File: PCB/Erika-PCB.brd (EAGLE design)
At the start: 100 x 80 mm, 11 parts

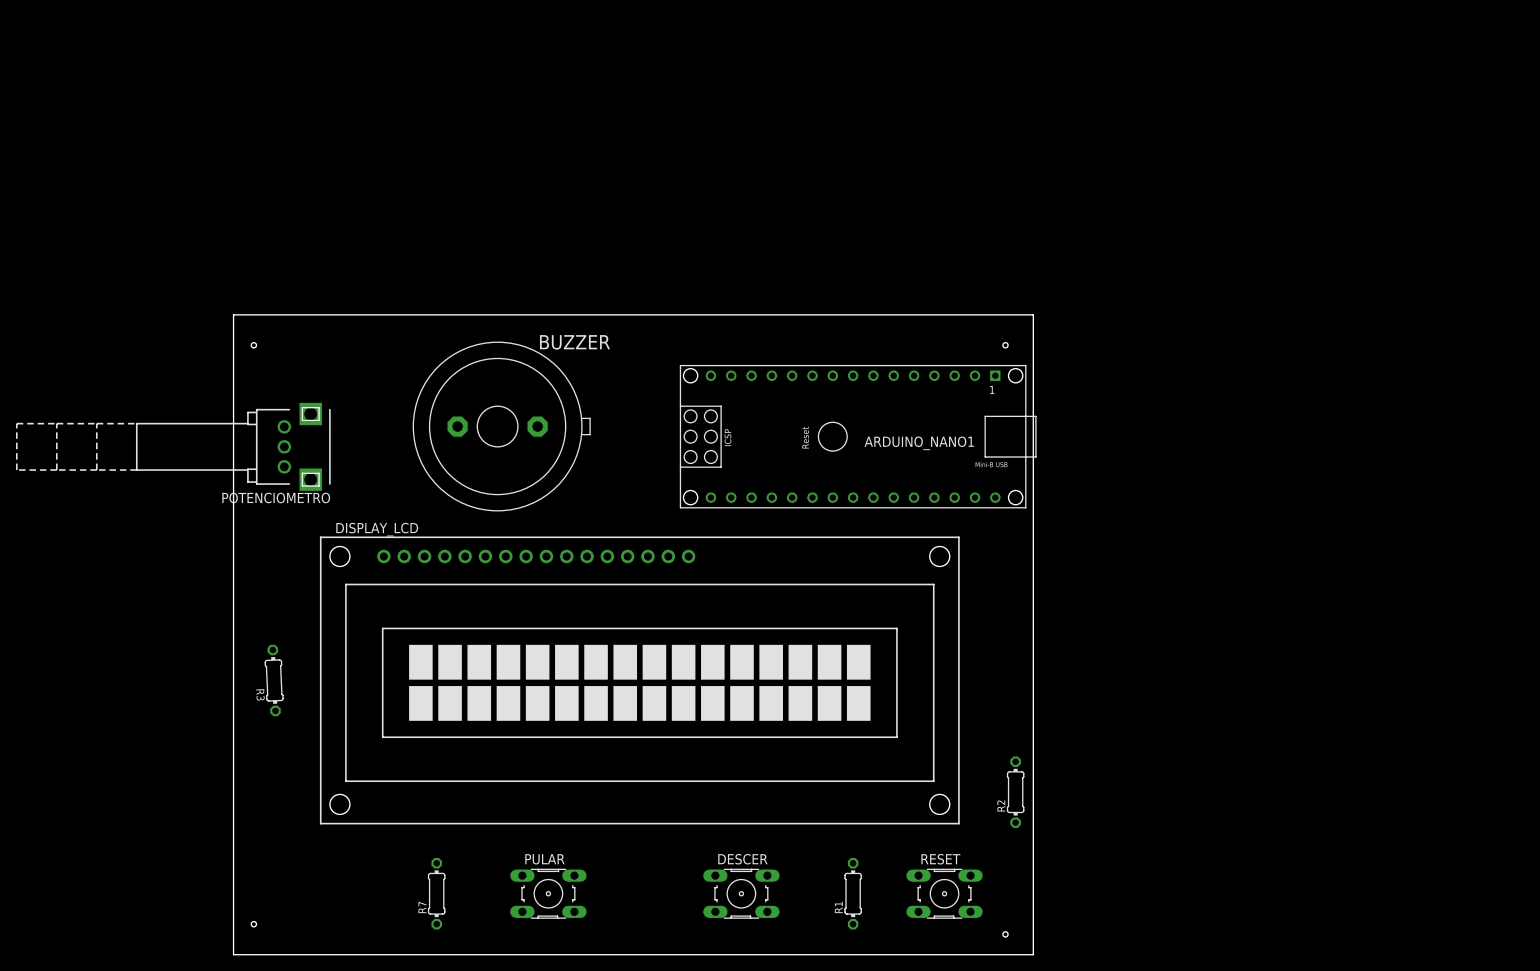
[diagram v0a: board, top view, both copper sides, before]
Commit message: Atualizando a PCB
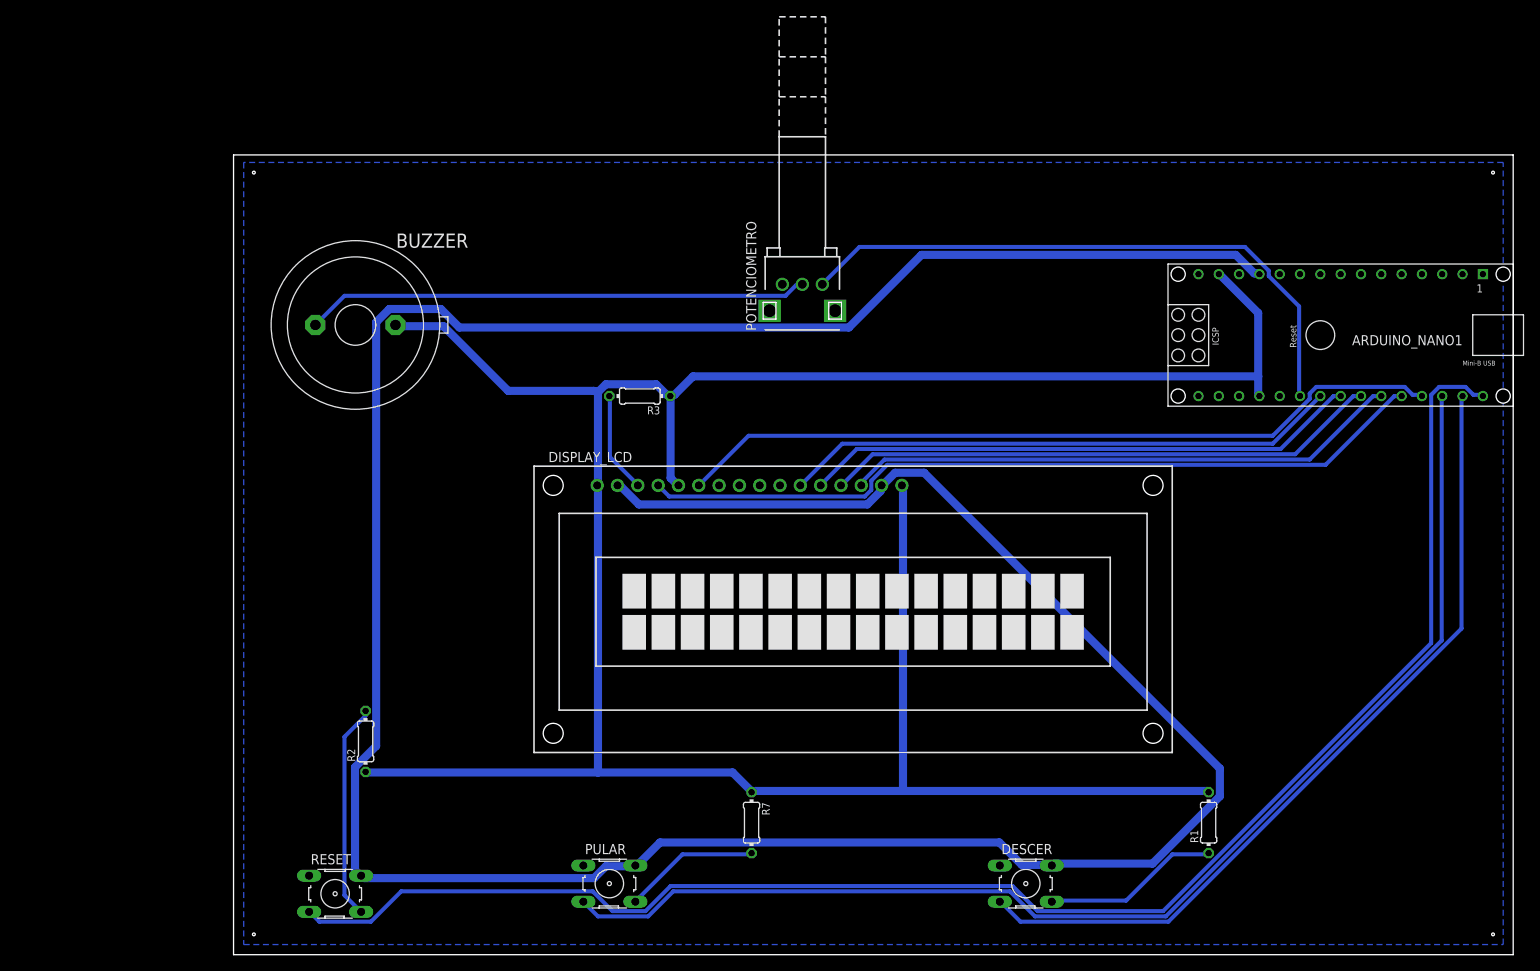
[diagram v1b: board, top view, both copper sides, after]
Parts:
- moved R2 81.5 mm to (16.5, 26.7)
- moved RESET 76.2 mm to (12.7, 7.62)
- moved POTENCIOMETRO 67.9 mm to (71.1, 83.8), turned to 90 degrees
- moved ARDUINO_NANO1 62.3 mm to (135.9, 77.5)
- moved R3 57.9 mm to (50.8, 69.8), turned to 180 degrees
- moved R1 45.3 mm to (121.9, 16.5)
- moved R7 40.4 mm to (64.8, 16.5), turned to 270 degrees
- moved DESCER 35.6 mm to (99.1, 8.89)
- moved DISPLAY_LCD 28.1 mm to (77.5, 43.2)
- moved BUZZER 21.8 mm to (15.2, 78.7)
- moved PULAR 7.73 mm to (47.0, 8.89)
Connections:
- net N$9 renamed VCC
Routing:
- net VCC: track 0.00 -> 398.6 mm
- net GND: track 0.00 -> 334.9 mm
- net N$5: track 0.00 -> 198.3 mm
- net N$3: track 0.00 -> 155.6 mm
- net N$4: track 0.00 -> 103.1 mm
- net N$14: track 0.00 -> 99.4 mm
- net N$15: track 0.00 -> 96.5 mm
- net N$16: track 0.00 -> 76.3 mm
- net N$13: track 0.00 -> 69.8 mm
- net N$7: track 0.00 -> 69.7 mm
- net N$1: track 0.00 -> 69.6 mm
- net N$12: track 0.00 -> 69.6 mm
- net N$6: track 0.00 -> 63.0 mm
- net N$8: track 0.00 -> 27.1 mm
- net N$2: track 0.00 -> 22.2 mm
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- added copper zone on layer 16, net GND
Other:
- board size 100 x 80 mm -> 160 x 100 mm
